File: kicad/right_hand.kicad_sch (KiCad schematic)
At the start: 29 parts, among them SW34 Gateron_ks_27, SW35 Gateron_ks_27, SW36 Gateron_ks_27, SW37 Gateron_ks_27, SW38 Gateron_ks_27, SW39 Gateron_ks_27, SW40 Gateron_ks_27, SW41 Gateron_ks_27, SW42 Gateron_ks_27, SW43 Gateron_ks_27, SW44 Gateron_ks_27, SW45 Gateron_ks_27, SW46 Gateron_ks_27, SW47 Gateron_ks_27, SW48 Gateron_ks_27, SW49 Gateron_ks_27, SW50 Gateron_ks_27, SW51 Gateron_ks_27, SW52 Gateron_ks_27, SW53 Gateron_ks_27, SW54 Gateron_ks_27, SW55 Gateron_ks_27, SW56 Gateron_ks_27, SW57 Gateron_ks_27, SW58 Gateron_ks_27, SW59 Gateron_ks_27, SW60 Gateron_ks_27, SW61 Gateron_ks_27, U3 74HC595

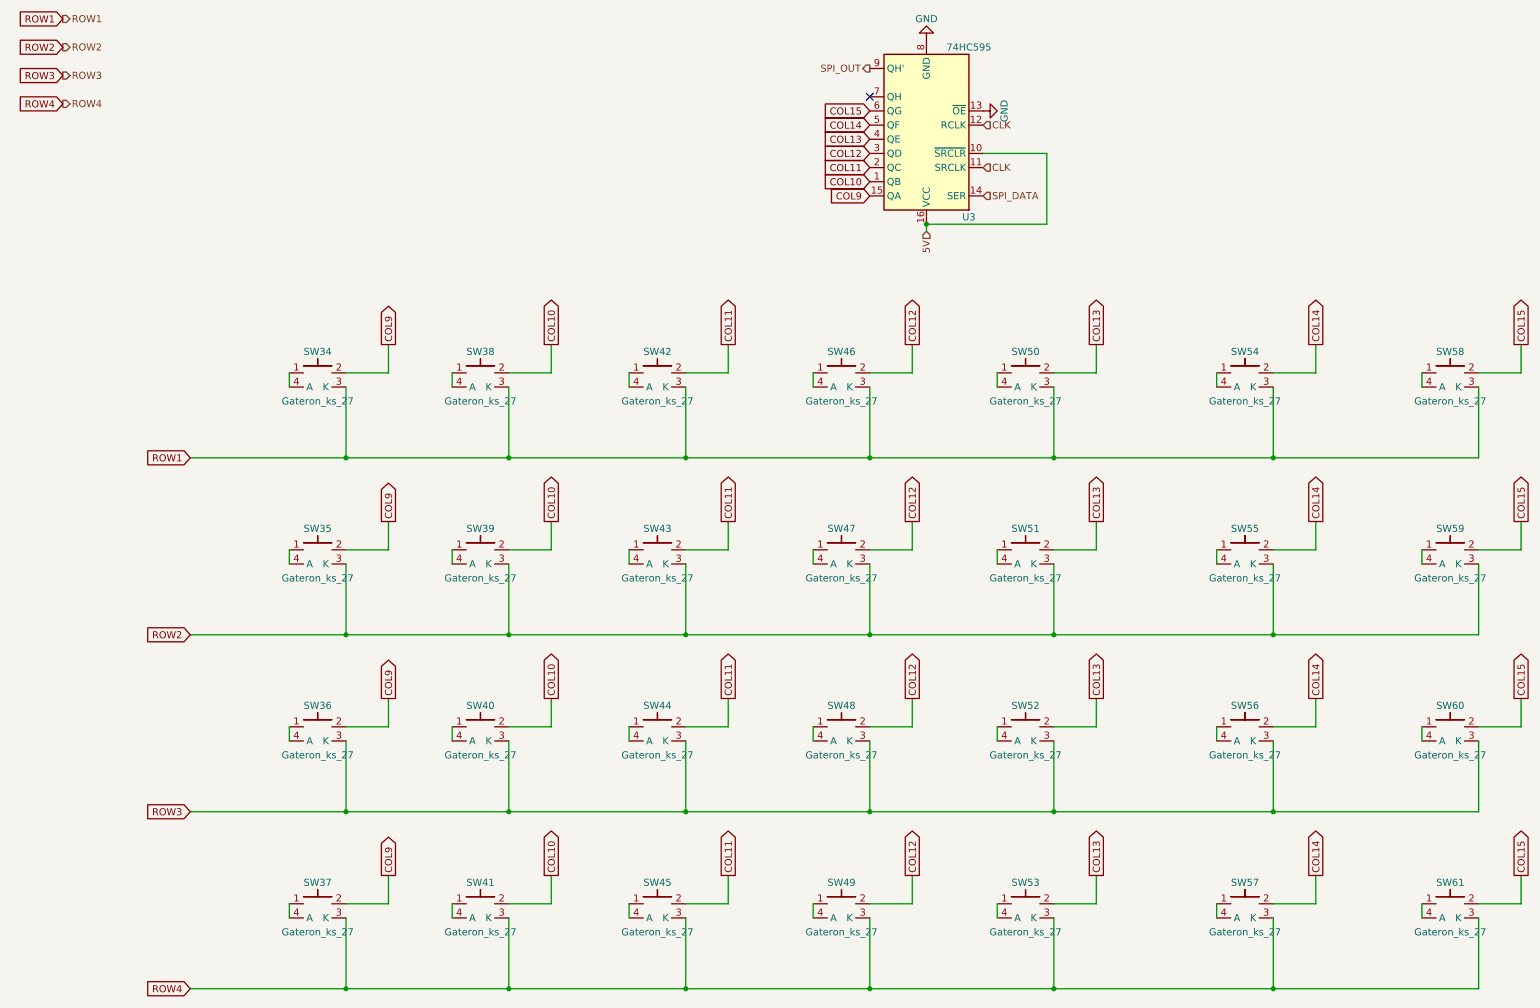
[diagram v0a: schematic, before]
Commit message: Update PCB
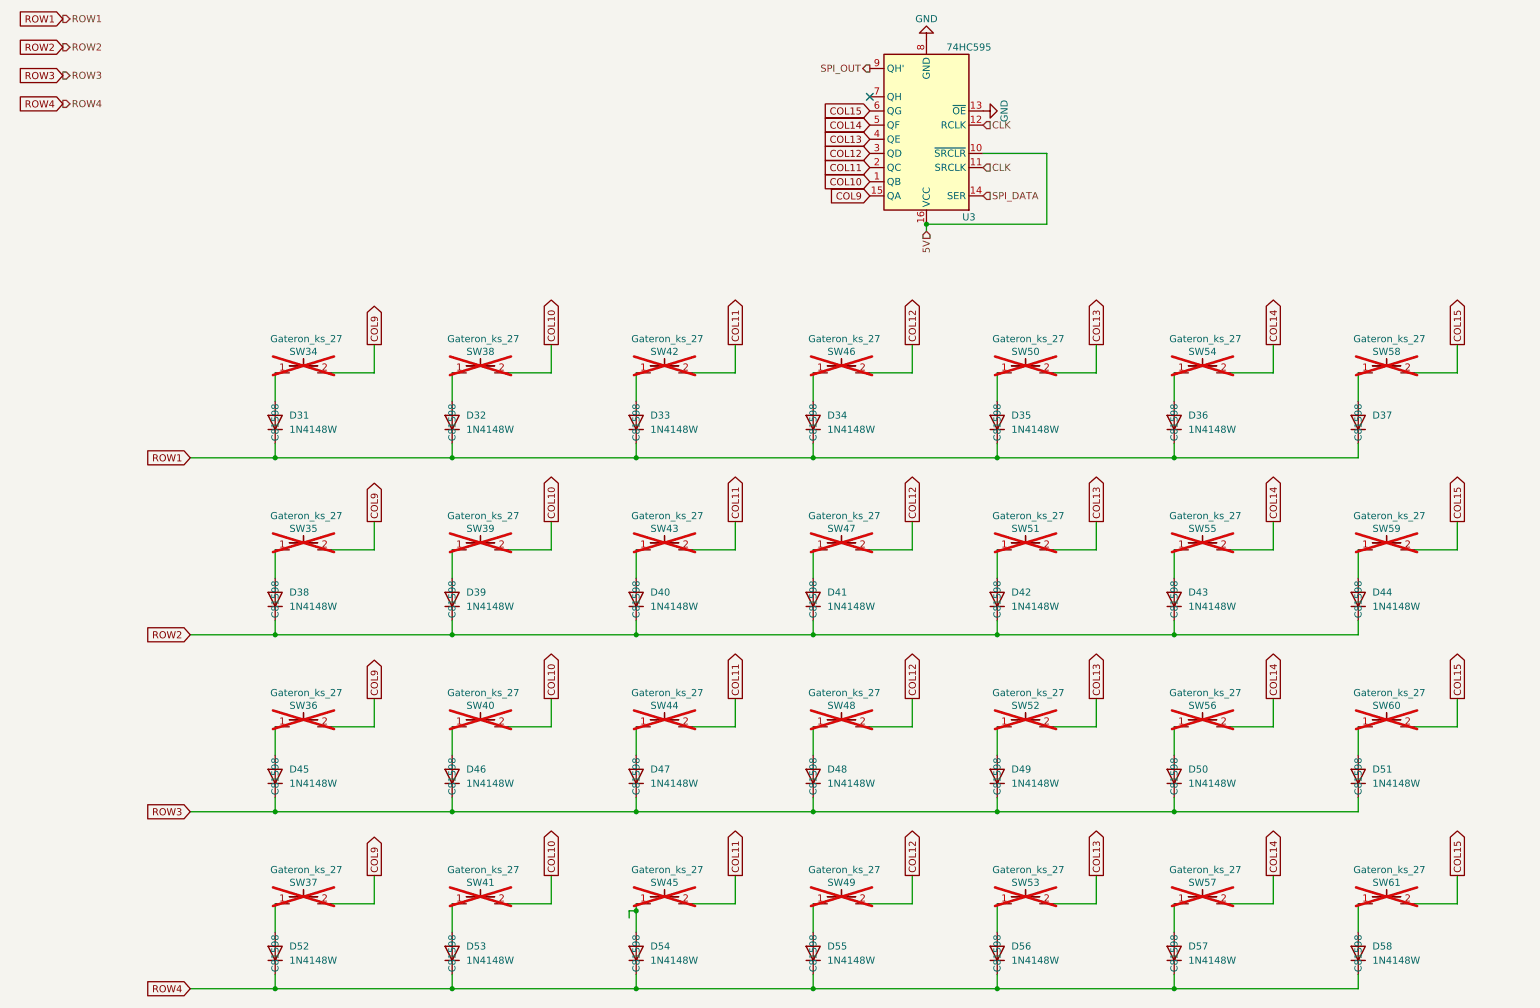
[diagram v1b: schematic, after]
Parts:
- added D31, D32, D33, D34, D35, D36, D37, D38, D39, D40, D41, D42, D43, D44, D45, D46, D47, D48, D49, D50, D51, D52, D53, D54, D55, D56, D57, D58: 1N4148W, Diode_SMD:D_SOD-123, symbol Diode:1N4148W-JLC
- SW34, SW35, SW36, SW37, SW38, SW39, SW40, SW41, SW42, SW43, SW44, SW45, SW46, SW47, SW48, SW49, SW50, SW51, SW52, SW53, SW54, SW55, SW56, SW57, SW58, SW59, SW60, SW61: now not fitted
- U3: LCSC (none) -> C72115
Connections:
- net ROW1: now also D31.1 (K), D32.1 (K), D33.1 (K), D34.1 (K), D35.1 (K), D36.1 (K), D37.1 (K); no longer SW34.3 (K), SW38.3 (K), SW42.3 (K), SW46.3 (K), SW50.3 (K), SW54.3 (K), SW58.3 (K)
- net ROW2: now also D38.1 (K), D39.1 (K), D40.1 (K), D41.1 (K), D42.1 (K), D43.1 (K), D44.1 (K); no longer SW35.3 (K), SW39.3 (K), SW43.3 (K), SW47.3 (K), SW51.3 (K), SW55.3 (K), SW59.3 (K)
- net ROW3: now also D45.1 (K), D46.1 (K), D47.1 (K), D48.1 (K), D49.1 (K), D50.1 (K), D51.1 (K); no longer SW36.3 (K), SW40.3 (K), SW44.3 (K), SW48.3 (K), SW52.3 (K), SW56.3 (K), SW60.3 (K)
- net ROW4: now also D52.1 (K), D53.1 (K), D54.1 (K), D55.1 (K), D56.1 (K), D57.1 (K), D58.1 (K); no longer SW37.3 (K), SW41.3 (K), SW45.3 (K), SW49.3 (K), SW53.3 (K), SW57.3 (K), SW61.3 (K)
- net at SW51.1: now also D42.2 (A); no longer SW51.4 (A)
- net at SW38.1: now also D32.2 (A); no longer SW38.4 (A)
- net at SW52.1: now also D49.2 (A); no longer SW52.4 (A)
- net at SW46.1: now also D34.2 (A); no longer SW46.4 (A)
- net at SW39.1: now also D39.2 (A); no longer SW39.4 (A)
- net at SW35.1: now also D38.2 (A); no longer SW35.4 (A)
- net at SW43.1: now also D40.2 (A); no longer SW43.4 (A)
- net at SW48.1: now also D48.2 (A); no longer SW48.4 (A)
- net at SW41.1: now also D53.2 (A); no longer SW41.4 (A)
- net at SW56.1: now also D50.2 (A); no longer SW56.4 (A)
- net at SW50.1: now also D35.2 (A); no longer SW50.4 (A)
- net at SW40.1: now also D46.2 (A); no longer SW40.4 (A)
- net at SW34.1: now also D31.2 (A); no longer SW34.4 (A)
- net at SW57.1: now also D57.2 (A); no longer SW57.4 (A)
- net at SW58.1: now also D37.2 (A); no longer SW58.4 (A)
- net at SW37.1: now also D52.2 (A); no longer SW37.4 (A)
- net at SW47.1: now also D41.2 (A); no longer SW47.4 (A)
- net at SW36.1: now also D45.2 (A); no longer SW36.4 (A)
- net at SW49.1: now also D55.2 (A); no longer SW49.4 (A)
- net at SW60.1: now also D51.2 (A); no longer SW60.4 (A)
- net at SW44.1: now also D47.2 (A); no longer SW44.4 (A)
- net at SW61.1: now also D58.2 (A); no longer SW61.4 (A)
- net at SW54.1: now also D36.2 (A); no longer SW54.4 (A)
- net at SW53.1: now also D56.2 (A); no longer SW53.4 (A)
- net at SW42.1: now also D33.2 (A); no longer SW42.4 (A)
- net at SW59.1: now also D44.2 (A); no longer SW59.4 (A)
- net at SW45.1: now also D54.2 (A); no longer SW45.4 (A)
- net at SW55.1: now also D43.2 (A); no longer SW55.4 (A)
